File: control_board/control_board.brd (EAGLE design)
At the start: 107.8 x 40 mm, 100 parts, among them IC1 TL072D

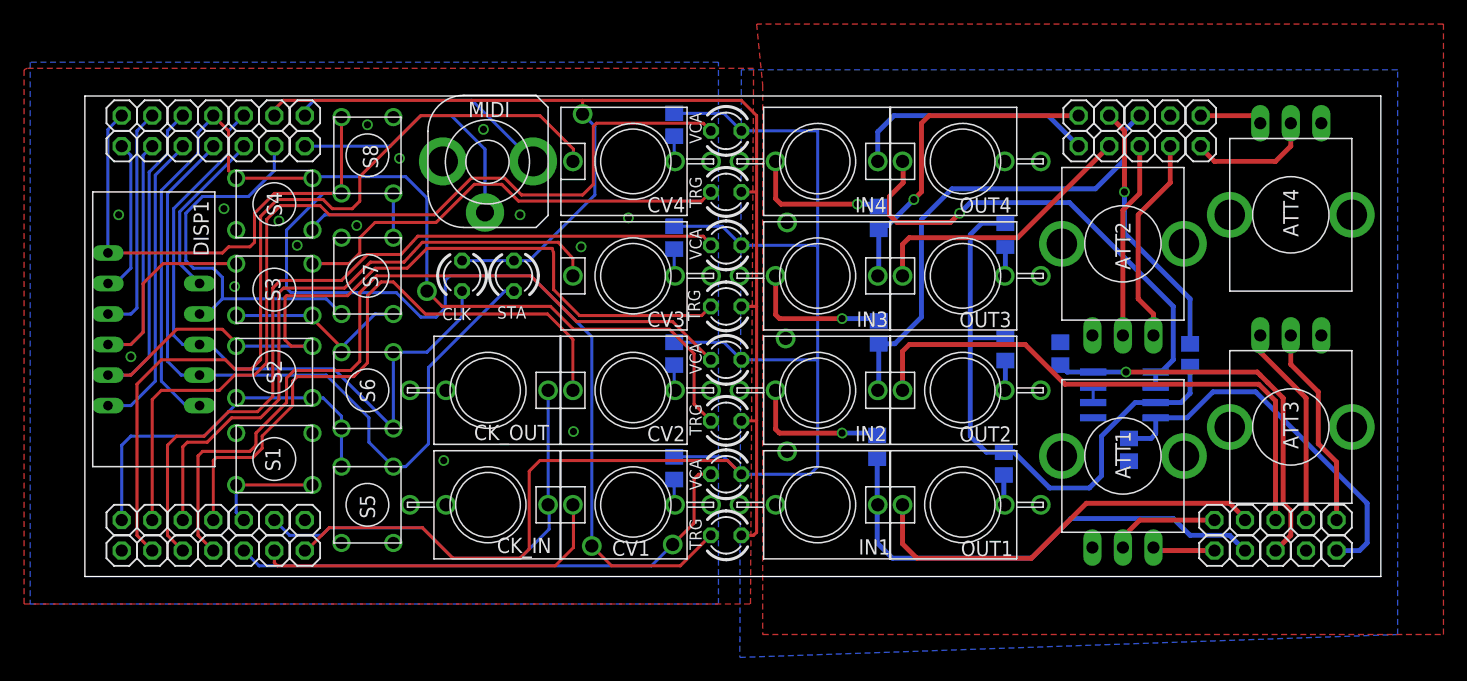
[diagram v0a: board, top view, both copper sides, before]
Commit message: fixes
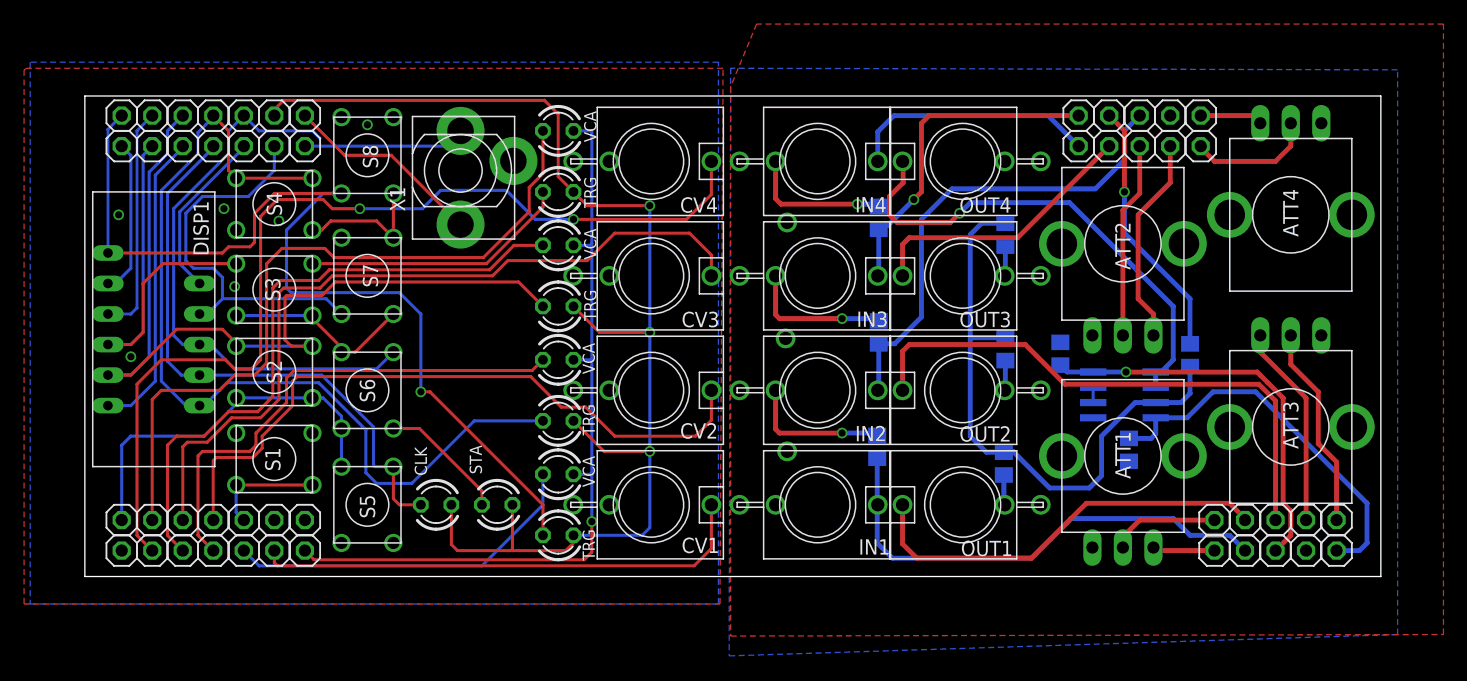
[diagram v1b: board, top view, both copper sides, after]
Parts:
- removed CK_IN, CK_OUT: WQP-PJ301M-12_JACK, thonkiconn:WQP-PJ301M-12_JACK
- removed MIDI: VERTICAL_3_5MM_SOCKET, jason_eagle6:VERTICAL_3_5MM_SOCKET
- removed R1, R2, R3, R4: (no value), rcl:R0805
- added X1: VERTICAL_3_5MM_SOCKETTHONK, jason_eagle6:PJ301CM
- moved LED9 20.1 mm to (41.9, 40.0), turned to 180 degrees
- moved LED10 19.3 mm to (47.0, 40.0), turned to 180 degrees
- moved LED_TRIG1 14.0 mm to (52.1, 56.5)
- moved LED_TRIG2 14.0 mm to (52.1, 66.0)
- moved LED_TRIG3 14.0 mm to (52.1, 37.5)
- moved LED_TRIG4 14.0 mm to (52.1, 47.0)
- moved LED_VCA1 14.0 mm to (52.1, 42.5)
- moved LED_VCA2 14.0 mm to (52.1, 52.1)
- moved LED_VCA3 14.0 mm to (52.1, 61.6)
- moved LED_VCA4 14.0 mm to (52.1, 71.1)
- moved CV1 1.52 mm to (59.8, 40.0), turned to 270 degrees
- moved CV2 1.52 mm to (59.8, 49.5), turned to 270 degrees
- moved CV3 1.52 mm to (59.8, 59.1), turned to 270 degrees
- moved CV4 1.52 mm to (59.8, 68.6), turned to 270 degrees
- turned DGND3 to 0 degrees
- renumbered CKIN to DGND3
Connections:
- removed net N$17: CK_IN.P$1, CK_OUT.P$1, DGND3.1
- removed net N$29: CV1.P$2, R1.2
- removed net N$30: CV2.P$2, R2.2
- removed net N$31: CV3.P$2, R3.2
- removed net N$32: CV4.P$2, R4.2
- net +5V: no longer R1.1, R2.1, R3.1, R4.1
- net GND: now also CV1.P$2, CV2.P$2, CV3.P$2, CV4.P$2, DGND3.1; no longer CK_IN.P$2, CK_IN.P$3, CK_OUT.P$3
- net N$19: now also X1.R; no longer MIDI.3
- net N$20: now also X1.T; no longer MIDI.4
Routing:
- net +5V: track 124.3 -> 65.7 mm, vias 0 -> 1
- net N$17: track 37.3 -> 0.00 mm
- net SINK3: track 112.1 -> 80.6 mm
- net N$22: track 65.3 -> 42.2 mm
- net SINK1: track 92.3 -> 73.5 mm
- net N$24: track 77.9 -> 60.5 mm
- net SINK2: track 72.5 -> 57.4 mm
- net N$23: track 67.4 -> 52.7 mm
- net N$21: track 44.7 -> 30.1 mm, vias 1 -> 0
- net SINK5: track 62.9 -> 48.9 mm
- net N$15: track 52.9 -> 65.1 mm
- net N$13: track 30.2 -> 41.7 mm
- net SINK4: track 89.0 -> 77.7 mm, vias 1 -> 0
- net N$16: track 71.6 -> 81.7 mm, vias 0 -> 2
- net N$19: track 22.5 -> 13.5 mm
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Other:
- board text added: "CONTROL BOARD V2"
